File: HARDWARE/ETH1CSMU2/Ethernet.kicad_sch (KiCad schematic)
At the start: 43 parts, among them U201 LAN8742A, U202 LC03-3.3, U203 LC03-3.3, Y201 NX5032GA-25.000000MHZ-LN-CD-1

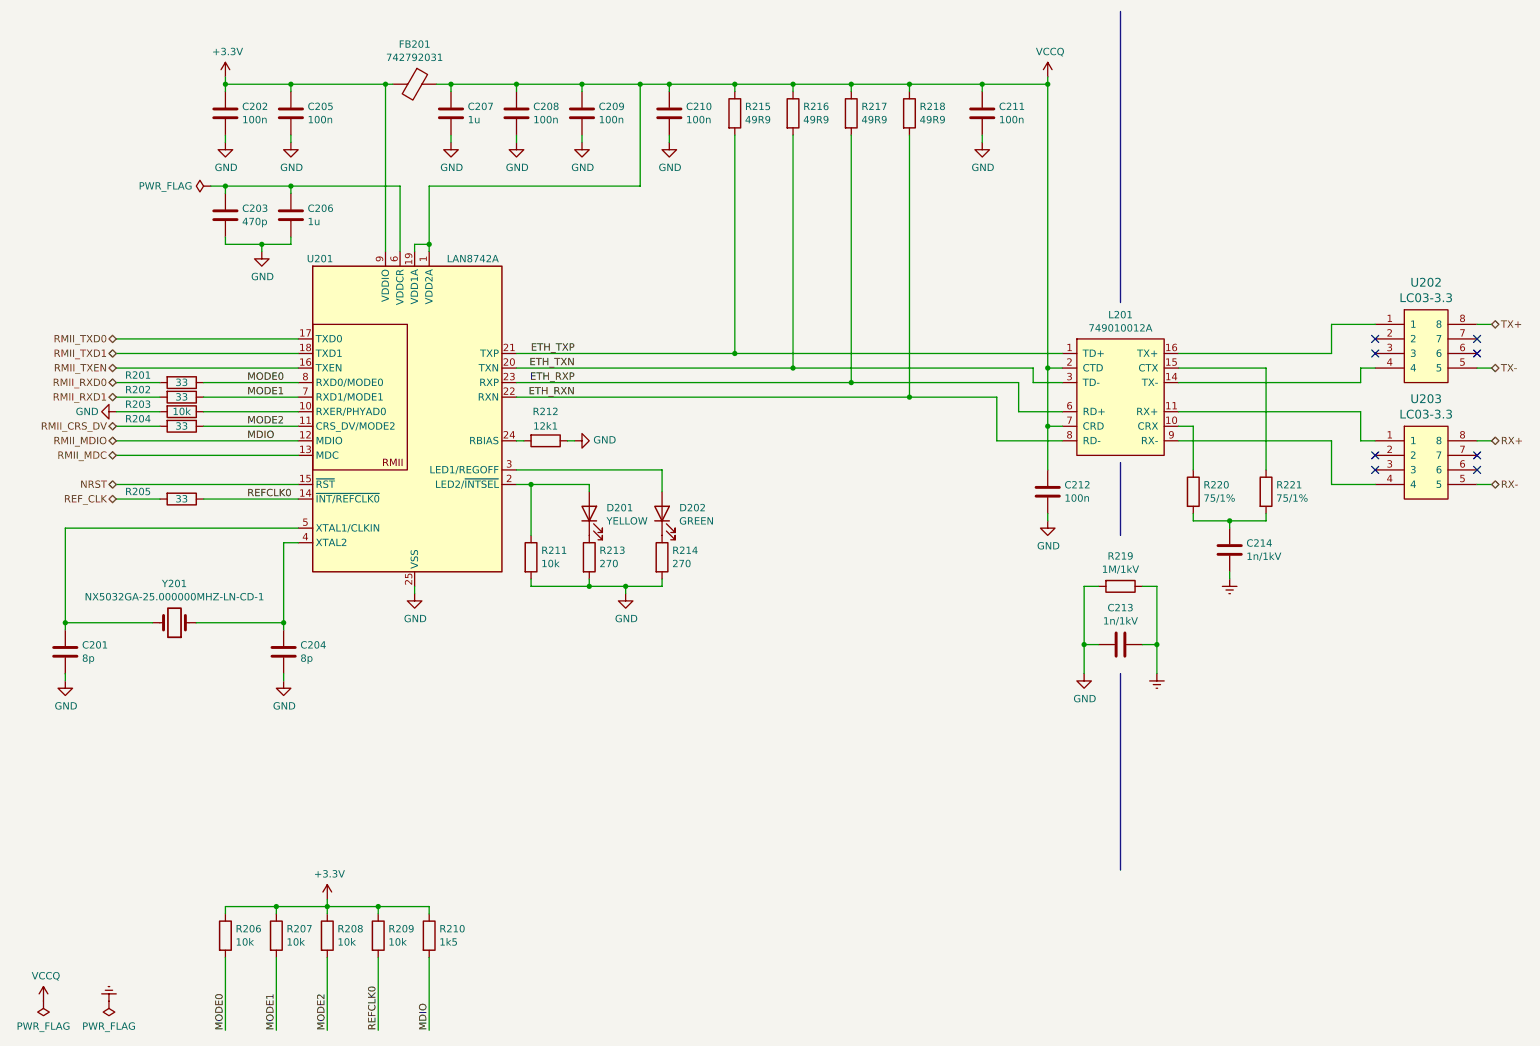
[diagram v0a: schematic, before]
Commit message: Hardware design
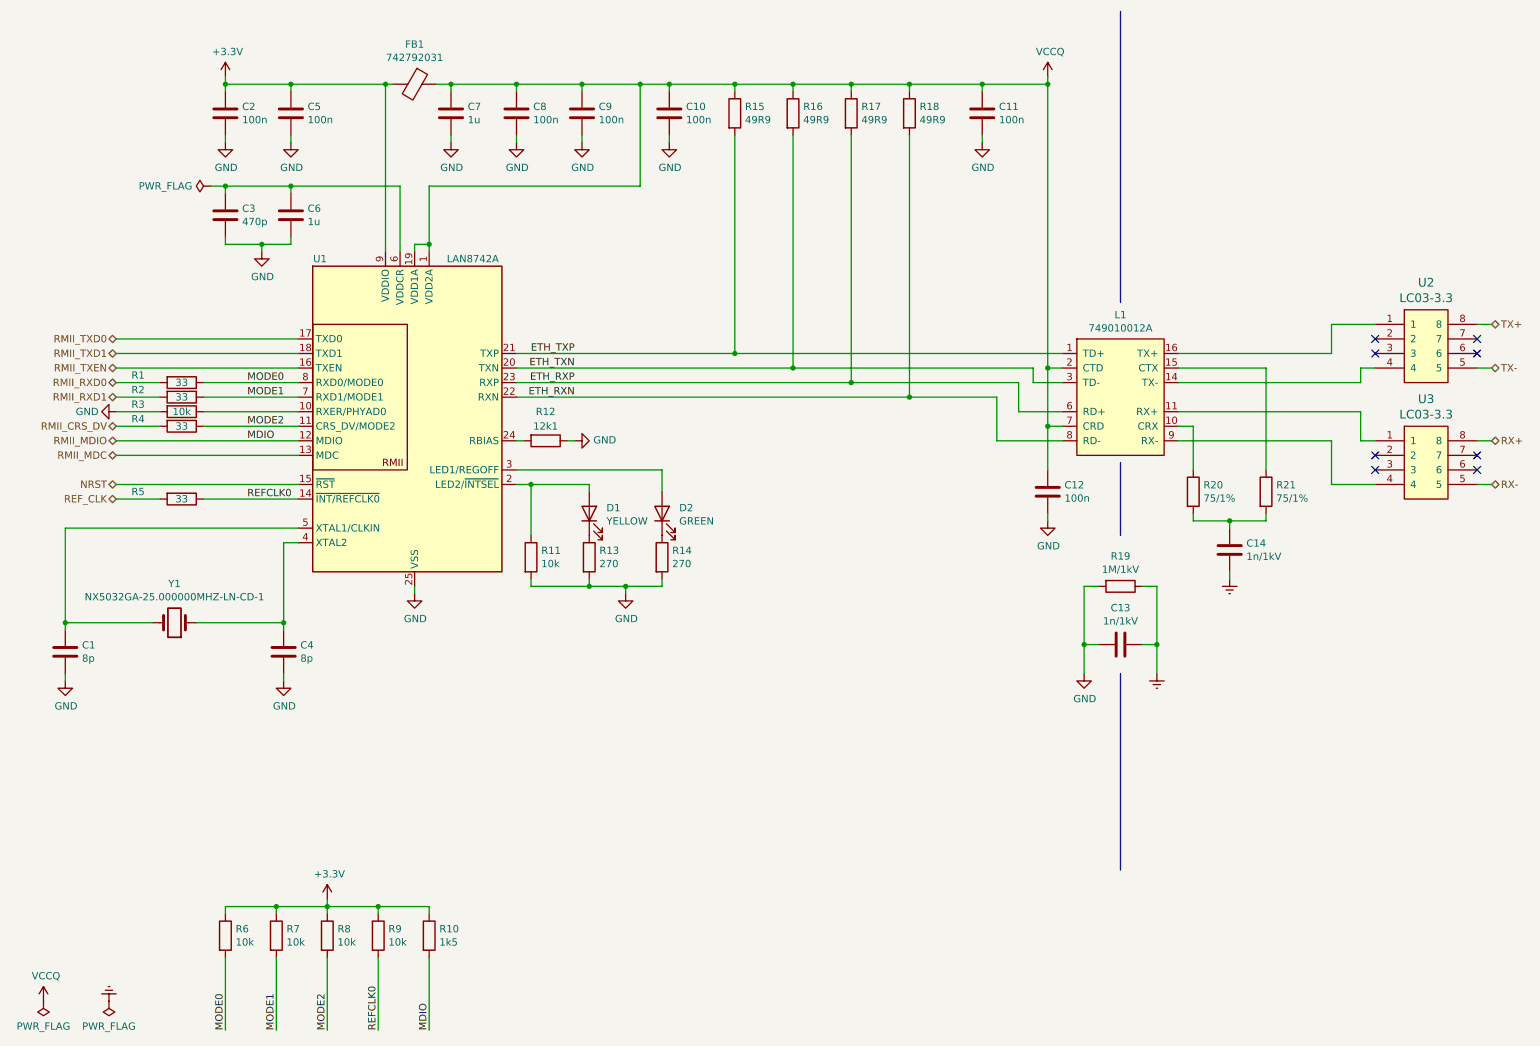
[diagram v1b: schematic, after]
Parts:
- renumbered C201 to C1, C210 to C10, C211 to C11, C212 to C12, C213 to C13, C214 to C14, C202 to C2, C203 to C3, C204 to C4, C205 to C5, C206 to C6, C207 to C7, C208 to C8, C209 to C9, D201 to D1, D202 to D2, FB201 to FB1, L201 to L1, R201 to R1, R210 to R10, R211 to R11, R212 to R12, R213 to R13, R214 to R14, R215 to R15, R216 to R16, R217 to R17, R218 to R18, R219 to R19, R202 to R2, R220 to R20, R221 to R21, R203 to R3, R204 to R4, R205 to R5, R206 to R6, R207 to R7, R208 to R8, R209 to R9, U201 to U1, U202 to U2, U203 to U3, Y201 to Y1

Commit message: Hardware design
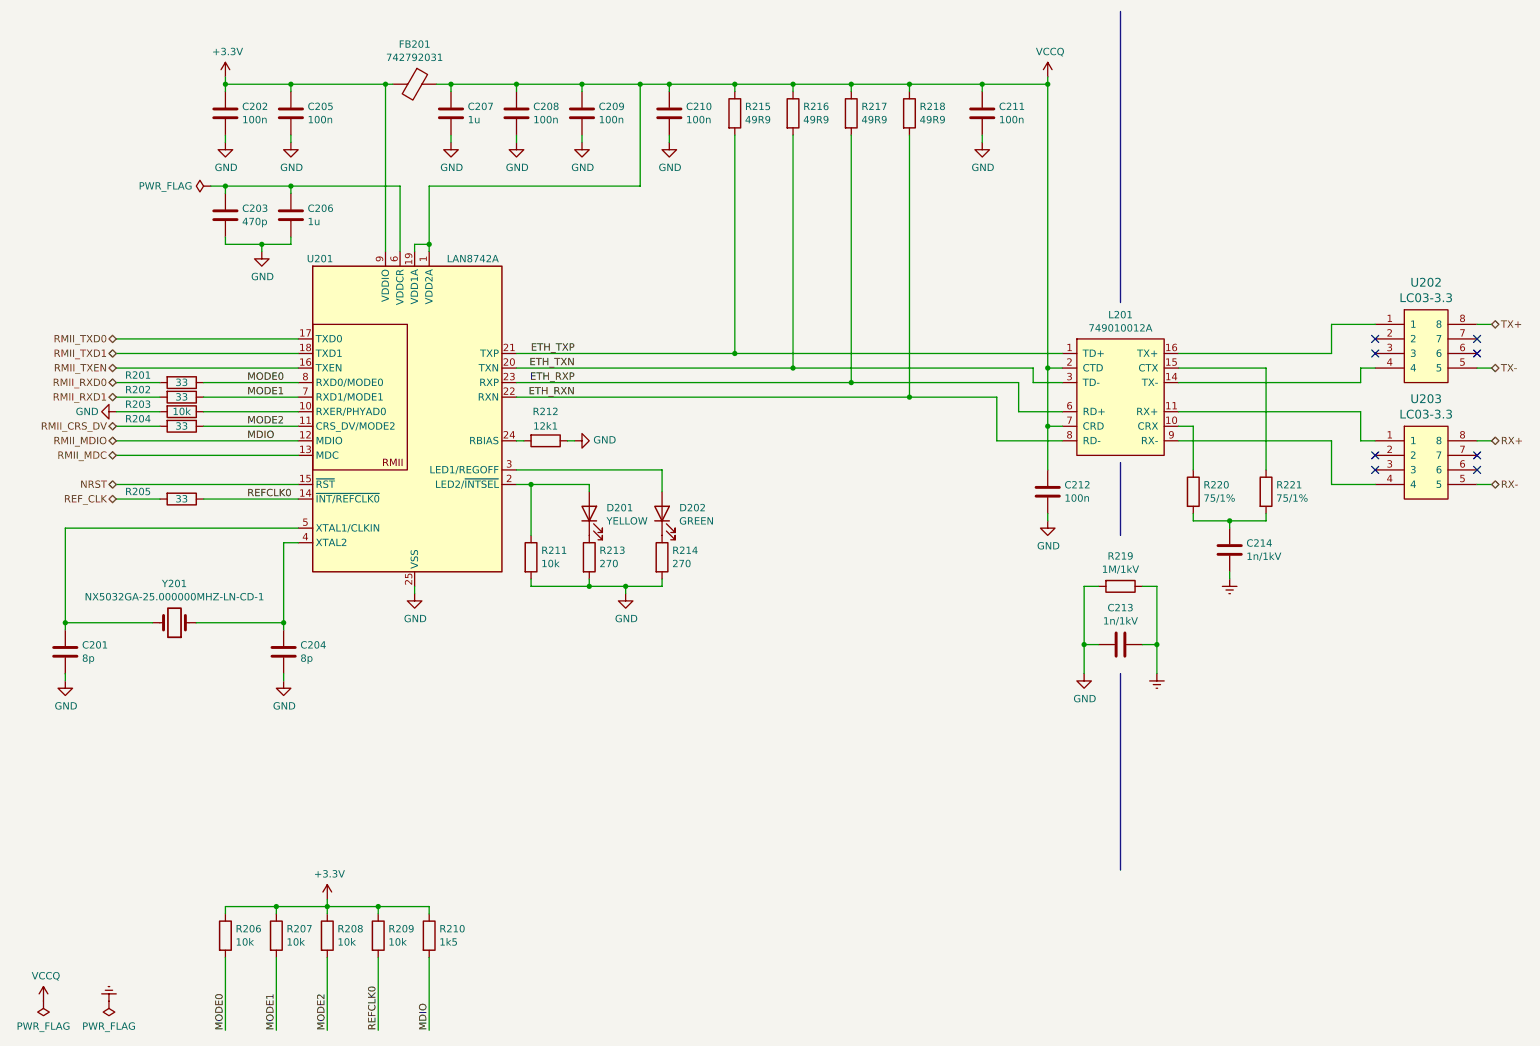
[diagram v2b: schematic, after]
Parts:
- renumbered C1 to C201, C2 to C202, C3 to C203, C4 to C204, C5 to C205, C6 to C206, C7 to C207, C8 to C208, C9 to C209, C10 to C210, C11 to C211, C12 to C212, C13 to C213, C14 to C214, D1 to D201, D2 to D202, FB1 to FB201, L1 to L201, R1 to R201, R2 to R202, R3 to R203, R4 to R204, R5 to R205, R6 to R206, R7 to R207, R8 to R208, R9 to R209, R10 to R210, R11 to R211, R12 to R212, R13 to R213, R14 to R214, R15 to R215, R16 to R216, R17 to R217, R18 to R218, R19 to R219, R20 to R220, R21 to R221, U1 to U201, U2 to U202, U3 to U203, Y1 to Y201
